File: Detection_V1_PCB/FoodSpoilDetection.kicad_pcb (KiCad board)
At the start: 2 copper layers, 60 x 65.2 mm, 44 parts, among them J1 Conn_01x03_Socket, J2 Conn_01x04_Socket, J3 Conn_01x06_Socket, J4 Conn_01x03_Socket, J5 Conn_01x10_Socket, J6 Conn_01x03_Socket, Q1 AO3401A, Q2 AO3400A, Q3 AO3401A, SW1 SW_DIP_x01, U1 XIAO-ESP32-S3-DIP

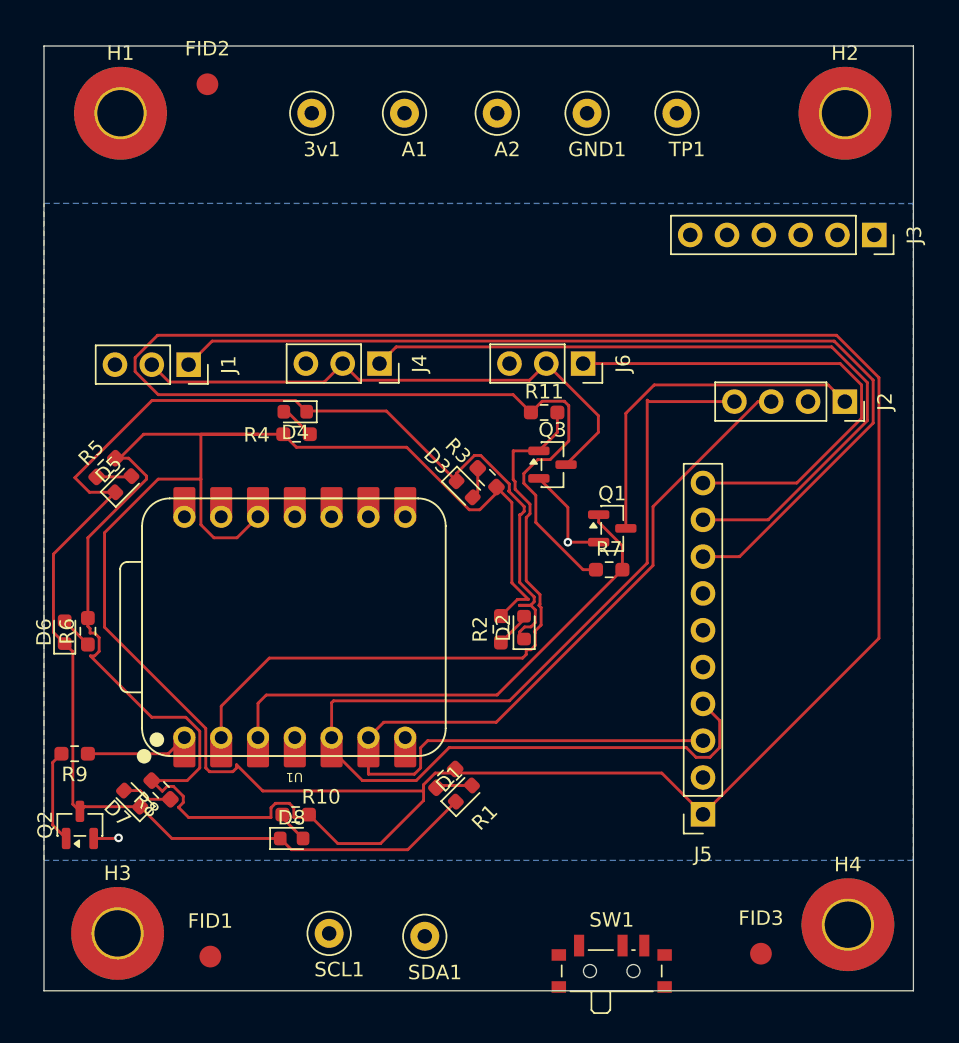
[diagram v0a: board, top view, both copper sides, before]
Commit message: measurements
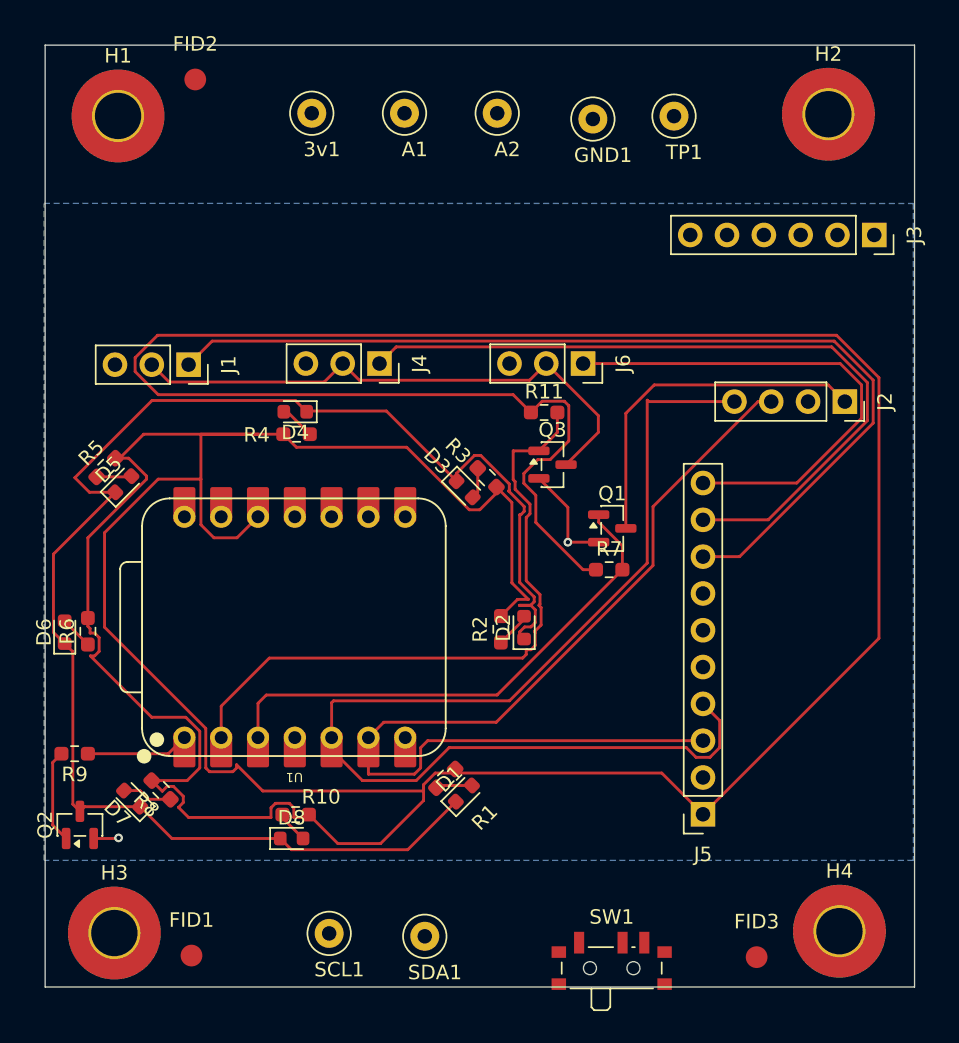
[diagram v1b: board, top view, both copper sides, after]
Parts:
- moved FID1 1.30 mm to (134.1, 131.7)
- moved H2 1.15 mm to (178.1, 73.7)
- moved FID2 0.90 mm to (134.4, 71.3)
- moved H4 0.74 mm to (178.8, 130.0)
- moved GND1 0.57 mm to (161.8, 74.0)
- moved FID3 0.38 mm to (173.1, 131.8)
- moved TP1 0.28 mm to (167.4, 73.8)
- moved H1 0.25 mm to (129.0, 73.8)
- moved H3 0.22 mm to (128.8, 130.2)
- moved SW1 0.20 mm to (163.1, 132.3)
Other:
- board size 60 x 65.2 mm -> 60 x 65 mm
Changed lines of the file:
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@@
 	(footprint "MountingHole:MountingHole_3.2mm_M3_Pad_TopBottom"
 		(layer "F.Cu")
-		(at 129 130.2)
+		(at 128.778 130.175)
 		(descr "Mounting Hole 3.2mm, M3, generated by kicad-footprint-generator mountinghole.py")
 		(tags "mountinghole M3")
@@
 	(footprint "Fiducial:Fiducial_1.5mm_Mask3mm"
 		(layer "F.Cu")
-		(at 173.4 131.6)
+		(at 173.101 131.84)
 		(descr "Fiducial, circular marking, 1.5mm bare copper, 3mm soldermask opening")
 		(tags "fiducial")
@@
 	(footprint "MountingHole:MountingHole_3.2mm_M3_Pad_TopBottom"
 		(layer "F.Cu")
-		(at 129.2 73.6)
+		(at 129.032 73.787)
 		(descr "Mounting Hole 3.2mm, M3, generated by kicad-footprint-generator mountinghole.py")
 		(tags "mountinghole M3")
@@
 	(footprint "Fiducial:Fiducial_1.5mm_Mask3mm"
 		(layer "F.Cu")
-		(at 135.2 71.6)
+		(at 134.36 71.27)
 		(descr "Fiducial, circular marking, 1.5mm bare copper, 3mm soldermask opening")
 		(tags "fiducial")
@@
 	(footprint "TestPoint:TestPoint_Loop_D1.80mm_Drill1.0mm_Beaded"
 		(layer "F.Cu")
-		(at 167.6 73.6)
+		(at 167.4 73.8)
 		(descr "wire loop with bead as test point, loop diameter 1.8mm, hole diameter 1.0mm")
 		(tags "test point wire loop bead")
@@
 	(footprint "MountingHole:MountingHole_3.2mm_M3_Pad_TopBottom"
 		(layer "F.Cu")
-		(at 179.2 73.6)
+		(at 178.054 73.67)
 		(descr "Mounting Hole 3.2mm, M3, generated by kicad-footprint-generator mountinghole.py")
 		(tags "mountinghole M3")
@@
 	(footprint "MountingHole:MountingHole_3.2mm_M3_Pad_TopBottom"
 		(layer "F.Cu")
-		(at 179.4 129.6)
+		(at 178.816 130.048)
 		(descr "Mounting Hole 3.2mm, M3, generated by kicad-footprint-generator mountinghole.py")
 		(tags "mountinghole M3")
@@
 	(footprint "Fiducial:Fiducial_1.5mm_Mask3mm"
 		(layer "F.Cu")
-		(at 135.4 131.8)
+		(at 134.1 131.73)
 		(descr "Fiducial, circular marking, 1.5mm bare copper, 3mm soldermask opening")
 		(tags "fiducial")
@@
 	(footprint "TestPoint:TestPoint_Loop_D1.80mm_Drill1.0mm_Beaded"
 		(layer "F.Cu")
-		(at 161.4 73.6)
+		(at 161.8 74)
 		(descr "wire loop with bead as test point, loop diameter 1.8mm, hole diameter 1.0mm")
 		(tags "test point wire loop bead")
@@
 	(footprint "Button_Switch_SMD:SW_SPDT_PCM12"
 		(layer "F.Cu")
-		(at 163.1 132.47)
+		(at 163.1 132.27)
 		(descr "Ultraminiature Surface Mount Slide Switch, right-angle, https://www.ckswitches.com/media/1424/pcm.pdf")
 		(property "Reference" "SW1"
@@
 	)
 	(gr_rect
-		(start 123.92 68.96)
-		(end 183.92 134.16)
+		(start 124 68.9)
+		(end 184 133.9)
 		(stroke
 			(width 0.05)
@@
 		(layer "Edge.Cuts")
 	)
+	(dimension
+		(type orthogonal)
+		(layer "F.Cu")
+		(pts
+			(xy 178.816 129.6) (xy 183.896 129.6)
+		)
+		(height 9.973)
+		(orientation 0)
+		(format
+			(prefix "")
+			(suffix "")
+			(units 3)
+			(units_format 0)
+			(precision 4)
+			(suppress_zeroes yes)
+		)
+		(style
+			(thickness 0.2)
+			(arrow_length 1.27)
+			(text_position_mode 0)
+			(arrow_direction outward)
+			(extension_height 0.58642)
+			(extension_offset 0.5)
+			(keep_text_aligned yes)
+		)
+		(gr_text "0.2"
+			(at 181.356 137.773 0)
+			(layer "F.Cu")
+			(effects
+				(font
+					(size 1.5 1.5)
+					(thickness 0.3)
+				)
+			)
+		)
+	)
+	(dimension
+		(type orthogonal)
+		(layer "F.Cu")
+		(pts
+			(xy 123.92 68.96) (xy 183.92 68.96)
+		)
+		(height -7.96)
+		(orientation 0)
+		(format
+			(prefix "")
+			(suffix "")
+			(units 3)
+			(units_format 0)
+			(precision 4)
+			(suppress_zeroes yes)
+		)
+		(style
+			(thickness 0.2)
+			(arrow_length 1.27)
+			(text_position_mode 0)
+			(arrow_direction outward)
+			(extension_height 0.58642)
+			(extension_offset 0.5)
+			(keep_text_aligned yes)
+		)
+		(gr_text "2.3622"
+			(at 153.92 59.2 0)
+			(layer "F.Cu")
+			(effects
+				(font
+					(size 1.5 1.5)
+					(thickness 0.3)
+				)
+			)
+		)
+	)
+	(dimension
+		(type orthogonal)
+		(layer "F.Cu")
+		(pts
+			(xy 183.92 68.96) (xy 183.92 134.16)
+		)
+		(height 9.68)
+		(orientation 1)
+		(format
+			(prefix "")
+			(suffix "")
+			(units 3)
+			(units_format 0)
+			(precision 4)
+			(suppress_zeroes yes)
+		)
+		(style
+			(thickness 0.2)
+			(arrow_length 1.27)
+			(text_position_mode 0)
+			(arrow_direction outward)
+			(extension_height 0.58642)
+			(extension_offset 0.5)
+			(keep_text_aligned yes)
+		)
+		(gr_text "2.5669"
+			(at 191.8 101.56 90)
+			(layer "F.Cu")
+			(effects
+				(font
+					(size 1.5 1.5)
+					(thickness 0.3)
+				)
+			)
+		)
+	)
 	(segment
